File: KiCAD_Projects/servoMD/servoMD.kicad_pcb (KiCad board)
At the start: 2 copper layers, 50 x 35 mm, 42 parts, among them P1 CONN_01X04, P2 CONN_01X03, P3 CONN_01X03, P4 CONN_01X03, P5 CONN_01X06, Q1 MOSFET_N, Q2 MOSFET_N, Q3 MOSFET_N, Q4 MOSFET_N, SW1 SW_PUSH, U1 STM32F103_48, U2 NCP1117ST33T3G, U3 PHTRANS, U4 NCP1117ST50T3G, U5 PHTRANS, U6 NCP5359, U7 NCP5359, X1 ceralock

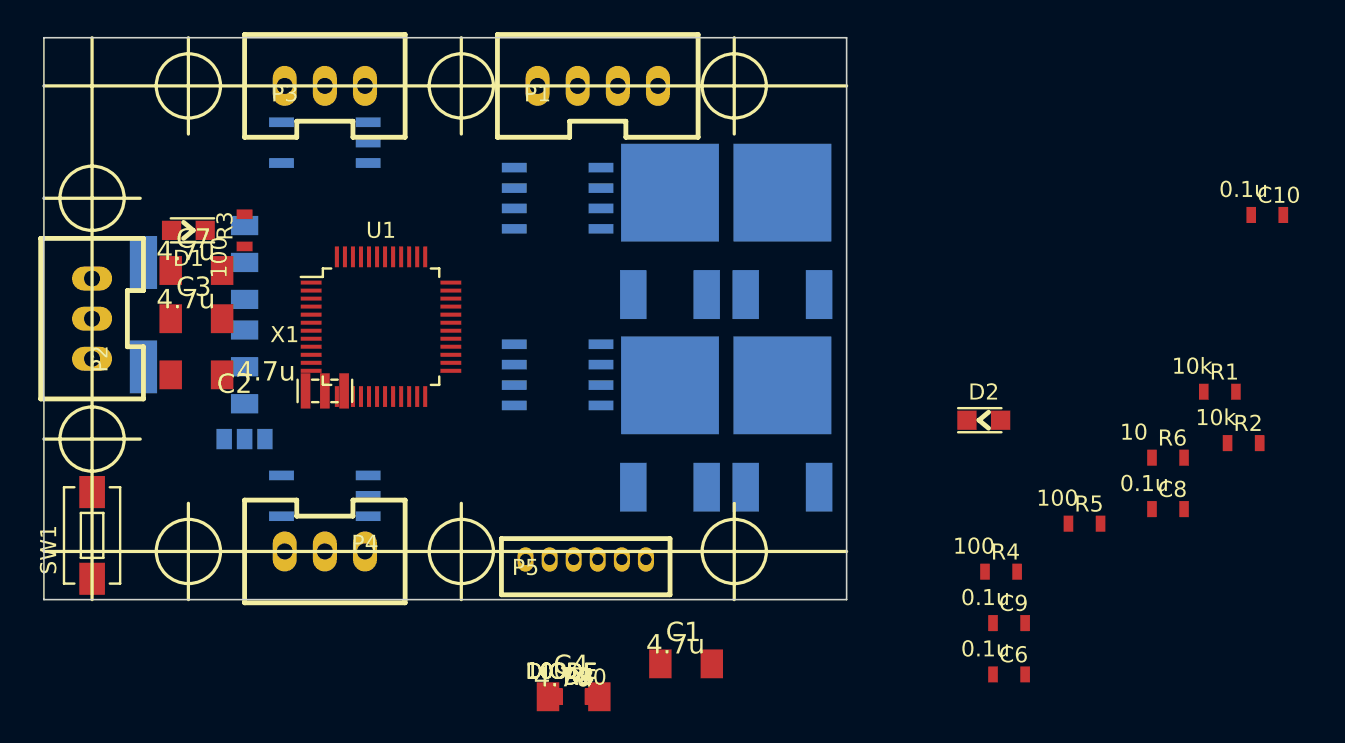
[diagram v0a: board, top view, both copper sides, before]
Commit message: 発注かけた
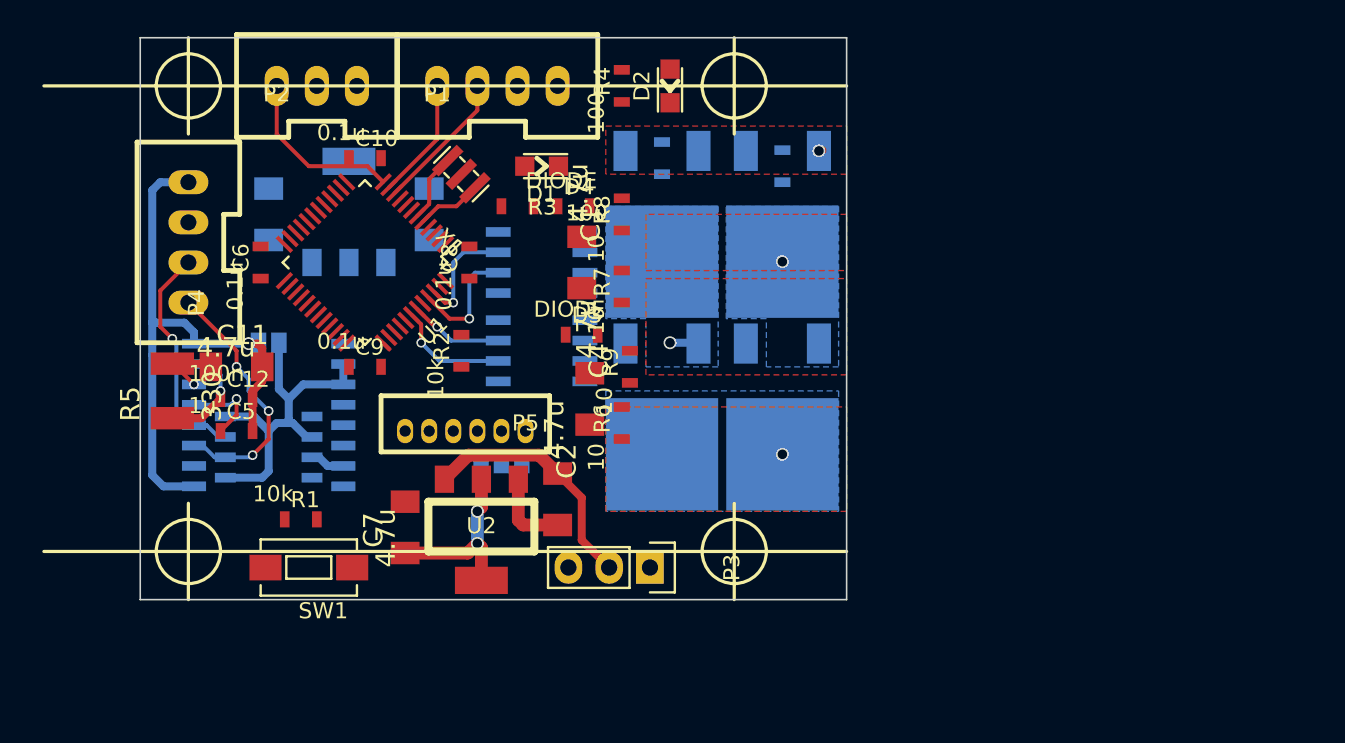
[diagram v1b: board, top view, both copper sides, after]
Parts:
- added C11: 4.7u, RP_KiCAD_Libs:C3216_S, F.Cu at (12.0, 20.5)
- added C12: 100n, RP_KiCAD_Libs:C1608_WP_S, F.Cu at (12.0, 22.5)
- added C13: 4.7u, RP_KiCAD_Libs:C3216_S, B.Cu at (24.0, 11.0)
- added C5: 1u, RP_KiCAD_Libs:C1608_WP_S, F.Cu at (12.0, 24.5)
- added JP1: JUMPER, Connect:GS2, B.Cu at (14.0, 19.0)
- added R11: 1k, RP_KiCAD_Libs:C1608_WP_S, B.Cu at (46.0, 8.00)
- C3: moved to B.Cu
- P3: footprint RP_KiCAD_Connector:XA_3T -> Pin_Headers:Pin_Header_Straight_1x03
- P4: value CONN_01X03 -> CONN_01X04; footprint RP_KiCAD_Connector:XA_3T -> RP_KiCAD_Connector:XA_4T
- Q1, Q2, Q3, Q4: footprint TO_SOT_Packages_SMD:TO-252-2Lead -> TO_SOT_Packages_SMD:SOT-428_GDS
- R10: value 100 -> 1k; moved to B.Cu
- R5: value 100 -> 330; footprint RP_KiCAD_Libs:C1608_WP_S -> RP_KiCAD_Libs:C3225
- U2: moved to F.Cu
- U3: value PHTRANS -> MAX3051; footprint RP_KiCAD_Libs:SOIC-5_3.9x4.9mm_Pitch1.27mm -> Housings_SOIC:SOIC-8_3.9x4.9mm_Pitch1.27mm_S
- U5: value PHTRANS -> ADM3052; footprint RP_KiCAD_Libs:SOIC-5_3.9x4.9mm_Pitch1.27mm -> Housings_SOIC:SOIC-16_7.5x10.3mm_Pitch1.27mm
- moved R1 57.8 mm to (16.0, 30.0)
- moved R5 57.4 mm to (8.00, 22.0), turned to 90 degrees
- moved C10 56.3 mm to (20.0, 7.50)
- moved C6 53.2 mm to (13.5, 14.0), turned to 90 degrees
- moved R2 49.1 mm to (26.0, 19.5), turned to 90 degrees
- moved C8 46.2 mm to (26.5, 14.0), turned to 90 degrees
- moved C9 43.2 mm to (20.0, 20.5)
- moved R4 38.4 mm to (36.0, 3.00), turned to 90 degrees
- moved P3 37.7 mm to (37.8, 33.0), turned to 270 degrees
- moved R6 34.1 mm to (36.0, 24.0), turned to 90 degrees
- moved R10 34.0 mm to (38.5, 7.50), turned to 270 degrees
- moved D4 30.6 mm to (33.0, 10.5)
- moved R8 30.2 mm to (36.0, 11.0), turned to 90 degrees
- moved D2 28.6 mm to (39.0, 3.00), turned to 90 degrees
- moved C1 25.8 mm to (33.5, 14.0), turned to 270 degrees
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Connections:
- P3 pad 1: GND -> +BATT
- P3 pad 3: Net-(P3-Pad3) -> /CAN_12V
- P4 pad 1: GND -> DGND
- P4 pad 2: +12V -> /CAN_12V
- P4 pad 3: Net-(P4-Pad3) -> /CAN_H
- R10 pad 1: Net-(P3-Pad3) -> GNDPWR
- R10 pad 2: Net-(R10-Pad2) -> Net-(C4-Pad1)
- R5 pad 1: Net-(R5-Pad1) -> Net-(C12-Pad1)
- R5 pad 2: Net-(R5-Pad2) -> Net-(C11-Pad1)
- R6 pad 1: (no net) -> Net-(Q1-PadG)
- R7 pad 1: (no net) -> Net-(Q2-PadG)
- R8 pad 1: (no net) -> Net-(Q3-PadG)
- R9 pad 1: (no net) -> Net-(Q4-PadG)
- U1 pad 21: Net-(R5-Pad2) -> (no net)
- U1 pad 22: Net-(U1-Pad22) -> (no net)
- U1 pad 32: (no net) -> /CAN_RX
- U1 pad 33: (no net) -> /CAN_TX
- U1 pad 42: (no net) -> /PWM_0
- U1 pad 43: (no net) -> /PWM_1
- U1 pad 45: (no net) -> /PWM_2
- U1 pad 46: (no net) -> /PWM_3
- U3 pad 1: Net-(R5-Pad1) -> /CAN_TX
- U3 pad 3: (no net) -> +3.3V
- U3 pad 4: GND -> /CAN_RX
- U3 pad 5: Net-(P4-Pad3) -> GND
- U3 pad 6: (no net) -> /CAN_L
- U5 pad 1: Net-(R10-Pad2) -> (no net)
- U5 pad 3: (no net) -> GND
- U5 pad 4: GND -> (no net)
- U5 pad 5: Net-(U1-Pad22) -> /CAN_RX
- U5 pad 6: +3.3V -> /CAN_TX
- U6 pad 2: (no net) -> /PWM_0
- U6 pad 3: (no net) -> /PWM_1
- U7 pad 2: (no net) -> /PWM_2
- U7 pad 3: (no net) -> /PWM_3
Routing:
- net DGND: track 0.00 -> 37.6 mm, vias 0 -> 1
- net GND: track 0.00 -> 27.6 mm
- net /CAN_L: track 0.00 -> 16.0 mm, vias 0 -> 3
- net +12V: track 0.00 -> 15.3 mm
- net /CAN_H: track 0.00 -> 14.4 mm, vias 0 -> 1
- net +5V: track 0.00 -> 11.3 mm, vias 0 -> 2
- net /POT: track 0.00 -> 10.9 mm
- net /ENC_A: track 0.00 -> 8.82 mm
- net /ENC_B: track 0.00 -> 7.58 mm
- net /PWM_2: track 0.00 -> 7.53 mm, vias 0 -> 1
- net /PWM_0: track 0.00 -> 7.27 mm, vias 0 -> 1
- net /PWM_3: track 0.00 -> 7.02 mm, vias 0 -> 1
- net Net-(C12-Pad1): track 0.00 -> 6.93 mm, vias 0 -> 1
- net /PWM_1: track 0.00 -> 5.86 mm, vias 0 -> 1
- net Net-(C5-Pad1): track 0.00 -> 5.22 mm, vias 0 -> 1
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- added copper zone on B.Cu, net +BATT
- added copper zone on F.Cu, net +BATT
- added copper zone on F.Cu, net GNDPWR
- added copper zone on B.Cu, net Net-(C1-Pad1)
- added copper zone on F.Cu, net Net-(C1-Pad1)
- added copper zone on B.Cu, net Net-(C4-Pad1)
- added copper zone on F.Cu, net Net-(C4-Pad1)
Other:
- board size 50 x 35 mm -> 44 x 35 mm
